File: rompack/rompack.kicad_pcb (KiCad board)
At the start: 2 copper layers, 65.2 x 41.5 mm, 4 parts, among them P1 CONN_MSXSLOT, U1 28C256

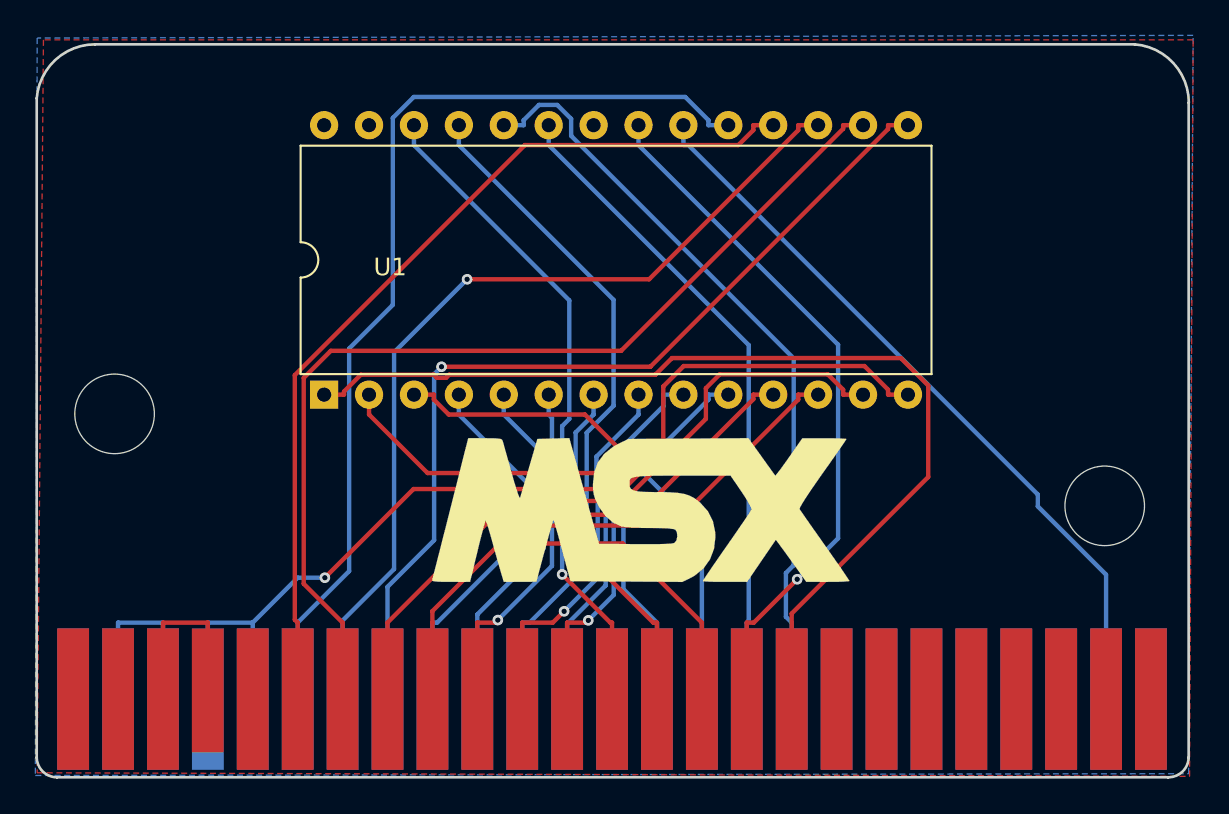
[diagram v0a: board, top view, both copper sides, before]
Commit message: many changes
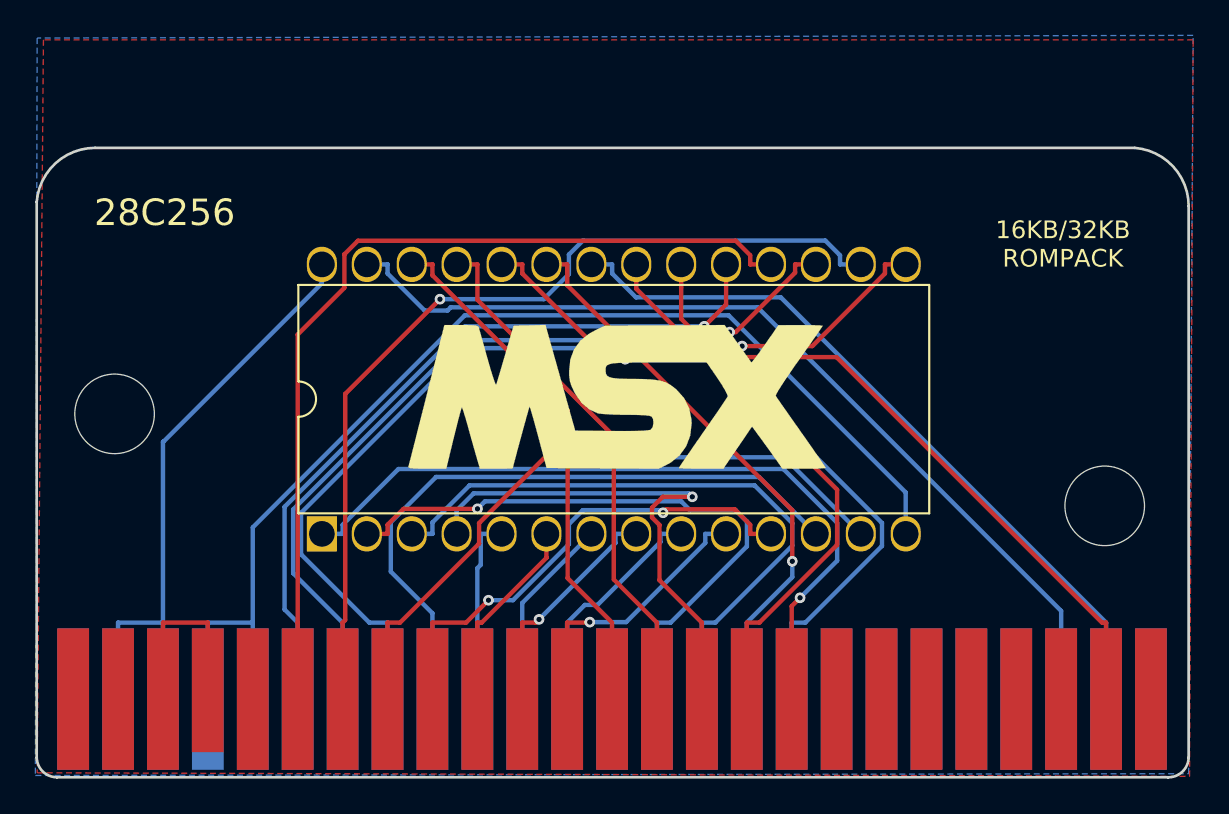
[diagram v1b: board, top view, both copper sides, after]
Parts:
- moved G*** 13.6 mm to (161.7, 91.3)
- moved U1 7.88 mm to (133.3, 98.8)
- moved G1 6.54 mm to (150.0, 91.1)
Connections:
- P1 pad 3: /SLTSL -> /CS12
- P1 pad 4: Net-(P1-Pad4) -> /SLTSL
- P1 pad 45: /5V0 -> VCC
- P1 pad 47: /5V0 -> VCC
- P1 pad 5: Net-(P1-Pad5) -> /WR0
- U1 pad 22: /RD -> /CS12
- U1 pad 27: Net-(U1-Pad27) -> /WR0
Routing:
- net /WR0: track 0.00 -> 55.3 mm
- net /CS12: track 0.00 -> 44.3 mm
- net VCC: track 0.00 -> 35.2 mm
- net /A14: track 56.9 -> 43.3 mm, vias 0 -> 1
- net /D7: track 55.4 -> 43.2 mm, vias 0 -> 1
- net /5V0: track 11.2 -> 0.00 mm
- net /A5: track 19.7 -> 10.6 mm
- net /A4: track 19.6 -> 11.1 mm, vias 1 -> 0
- net /A8: track 38.5 -> 30.0 mm, vias 1 -> 0
- net /A3: track 19.1 -> 11.0 mm
- net /A2: track 21.0 -> 13.2 mm
- net GND: track 57.2 -> 65.0 mm, vias 1 -> 0
- net /A10: track 39.5 -> 31.8 mm, vias 1 -> 0
- net /A1: track 20.7 -> 13.1 mm
- net /A0: track 23.2 -> 15.7 mm
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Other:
- board size 65.2 x 41.5 mm -> 65.2 x 35.6 mm
- board text added: "16KB/32KB ROMPACK"
- board text added: "2019.1.21"
- board text added: "28C256"
- board text added: "meeso.kim@gmail.com"
- board text removed: "2018.9.12"
